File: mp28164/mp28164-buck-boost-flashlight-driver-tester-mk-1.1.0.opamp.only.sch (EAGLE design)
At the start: 13 parts, among them U3 OPA333

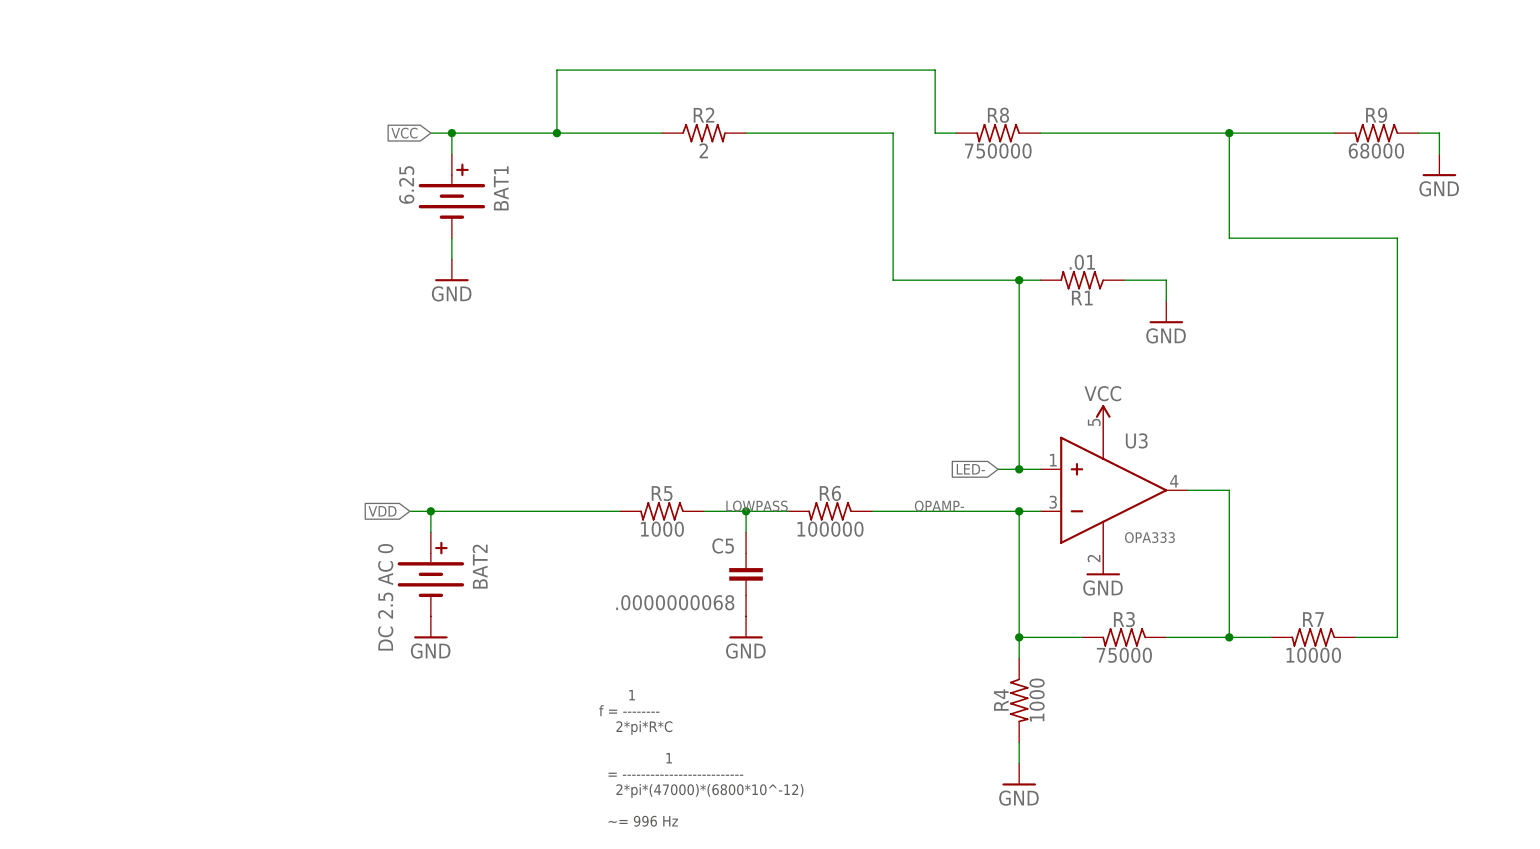
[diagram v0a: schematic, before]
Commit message: whole bunch of crap in here
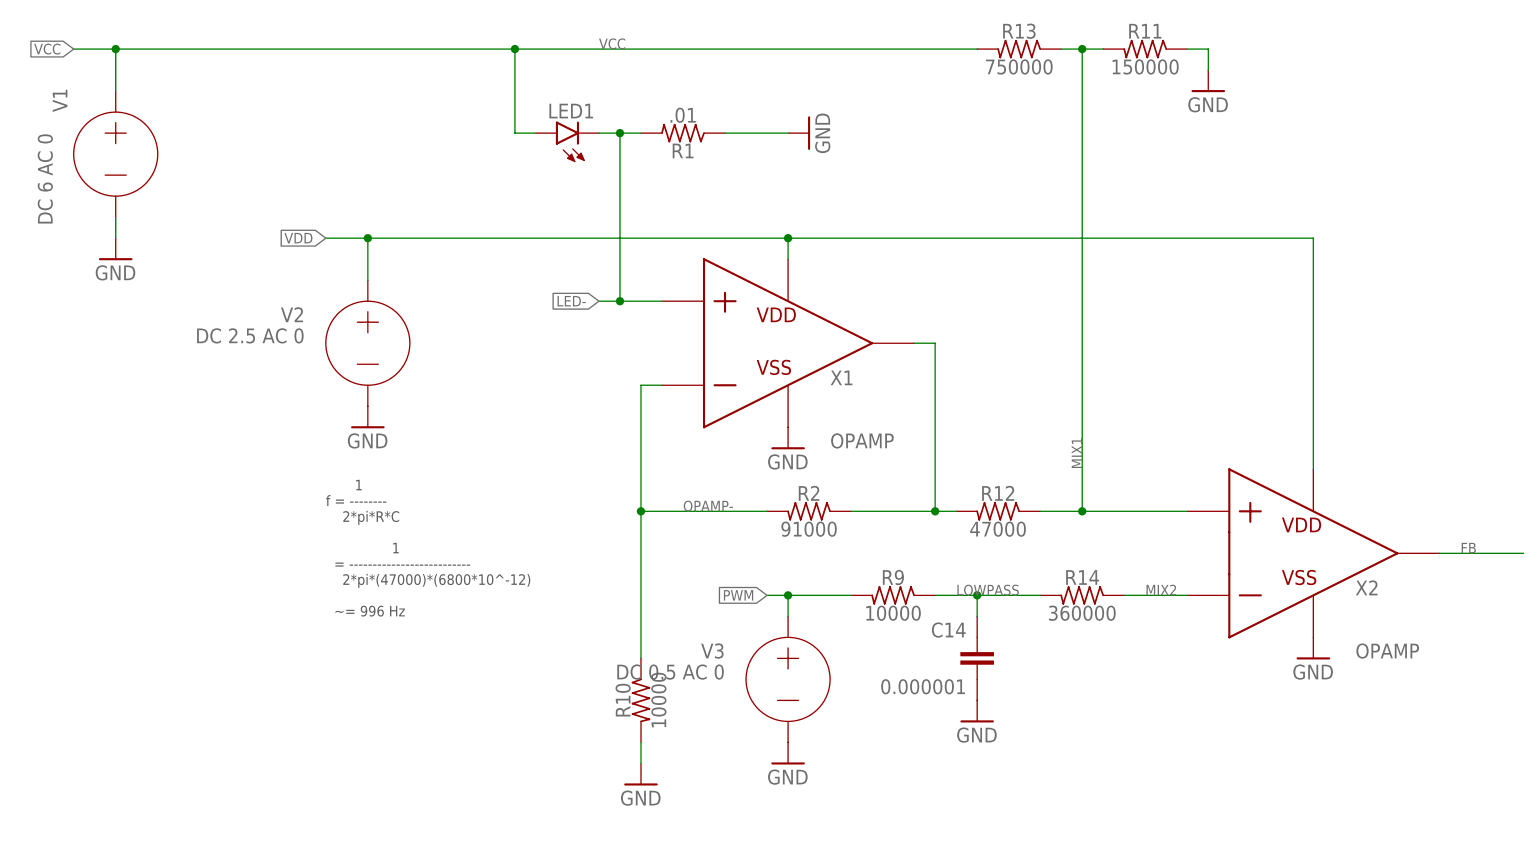
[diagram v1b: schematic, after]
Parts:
- removed BAT1: 6.25, a_parts:BATTERY9V
- removed BAT2: DC 2.5 AC 0, a_parts:BATTERY9V
- removed C5: .0000000068, a_parts:CAPACITOR-CERAMICC0402
- removed R3: 75000, a_parts:RESISTORR0402
- removed R4, R5: 1000, a_parts:RESISTORR0402
- removed R6: 100000, a_parts:RESISTORR0402
- removed R7: 10000, a_parts:RESISTORR0402
- removed R8: 750000, a_parts:RESISTORR0402
- removed U3: OPA333, a_parts:OPAMPOPA333-SC-70
- added C14: 0.000001, a_parts:CAPACITOR-CERAMICC0402
- added LED1: LED3MM, a_parts:LED3MM
- added R10: 10000, a_parts:RESISTORR0402
- added R11: 150000, a_parts:RESISTORR0402
- added R12: 47000, a_parts:RESISTORR0402
- added R13: 750000, a_parts:RESISTORR0402
- added R14: 360000, a_parts:RESISTORR0402
- added V1: DC 6 AC 0, ngspice-simulation:VOLTAGE
- added V2: DC 2.5 AC 0, ngspice-simulation:VOLTAGE
- added V3: DC 0.5 AC 0, ngspice-simulation:VOLTAGE
- added X1, X2: OPAMP, ngspice-simulation:OPAMP
- R2: value 2 -> 91000; device a_parts:RESISTOR0204/2V -> a_parts:RESISTORR0402
- R9: value 68000 -> 10000
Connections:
- removed net N$2: R7.1, R8.1, R9.2
- new net FB: X2.VOUT
- new net MIX1: R11.2, R12.1, R13.1, X2.P
- new net MIX2: R14.1, X2.N
- new net PWM: R9.2, V3.+
- net GND: now also C14.2, R10.2, R11.1, V1.-, V2.-, V3.-, X1.VSS, X2.VSS; no longer BAT1.-, BAT2.-, C5.2, R4.2, R9.1, U3.V-
- net LED-: now also LED1.C, X1.P; no longer R2.2, U3.IN+
- net LOWPASS: now also C14.1, R14.2, R9.1; no longer C5.1, R5.1, R6.2
- net OPAMP-: now also R10.1, R2.2, X1.N; no longer R3.2, R4.1, R6.1, U3.IN-
- net OPAMP_OUT: now also R12.2, R2.1, X1.VOUT; no longer R3.1, R7.2, U3.OUT
- net VCC: now also LED1.A, R13.2, V1.+; no longer BAT1.+, R2.1, R8.2, U3.V+
- net VDD: now also V2.+, X1.VDD, X2.VDD; no longer BAT2.+, R5.2
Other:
- moved on the sheet: R1, R2, R9
